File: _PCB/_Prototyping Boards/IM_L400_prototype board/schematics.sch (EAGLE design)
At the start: 10 parts

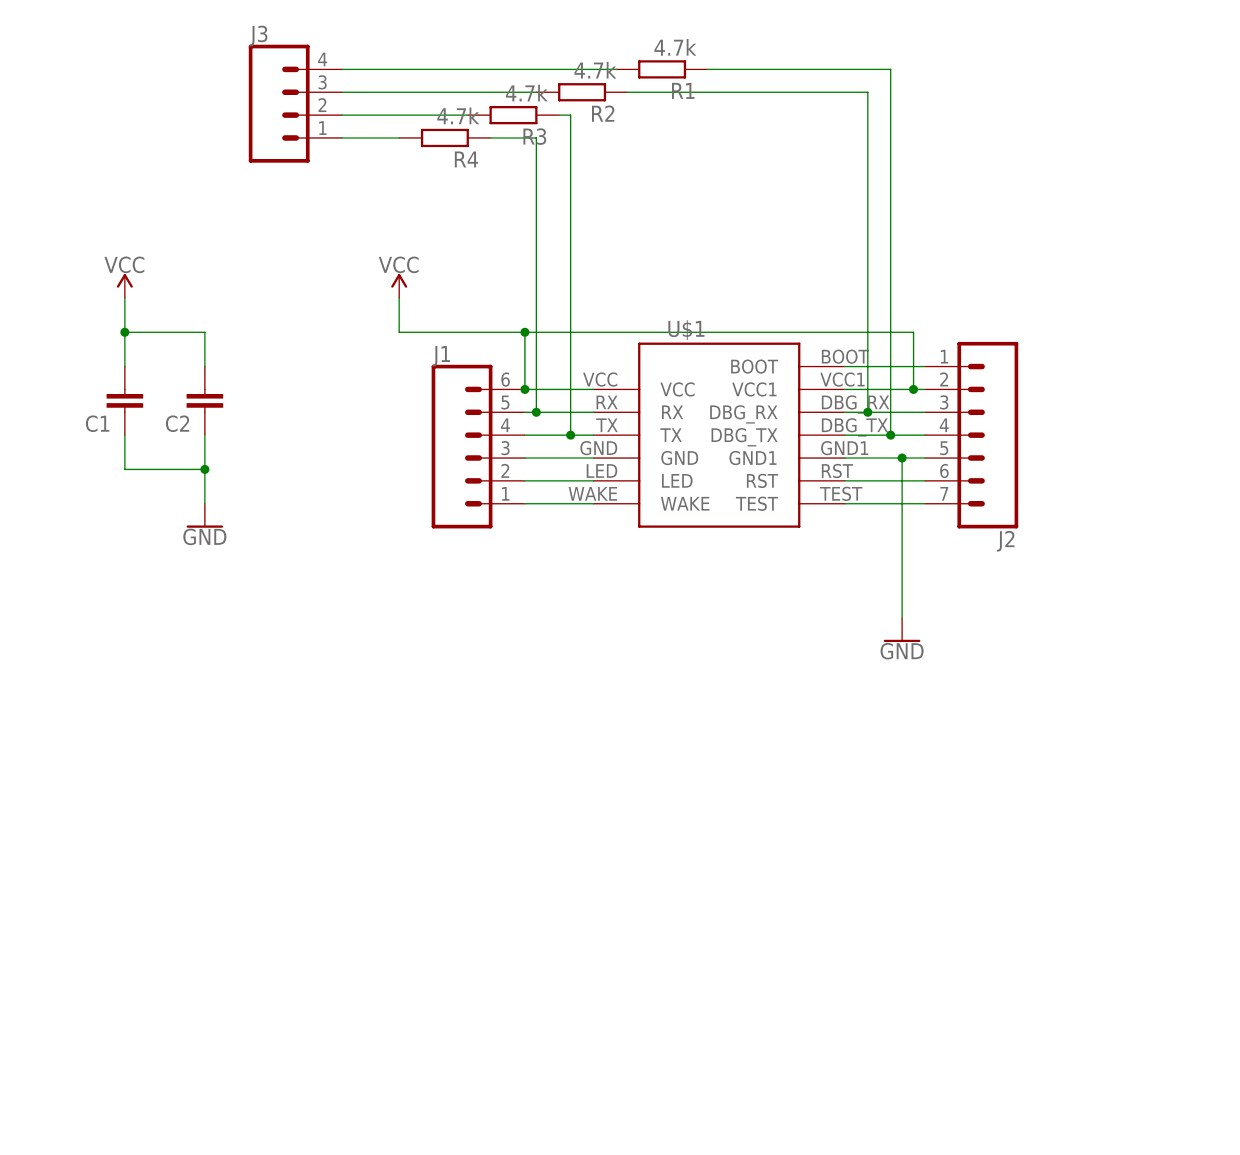
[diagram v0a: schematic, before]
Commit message: IM-L400 prototype board
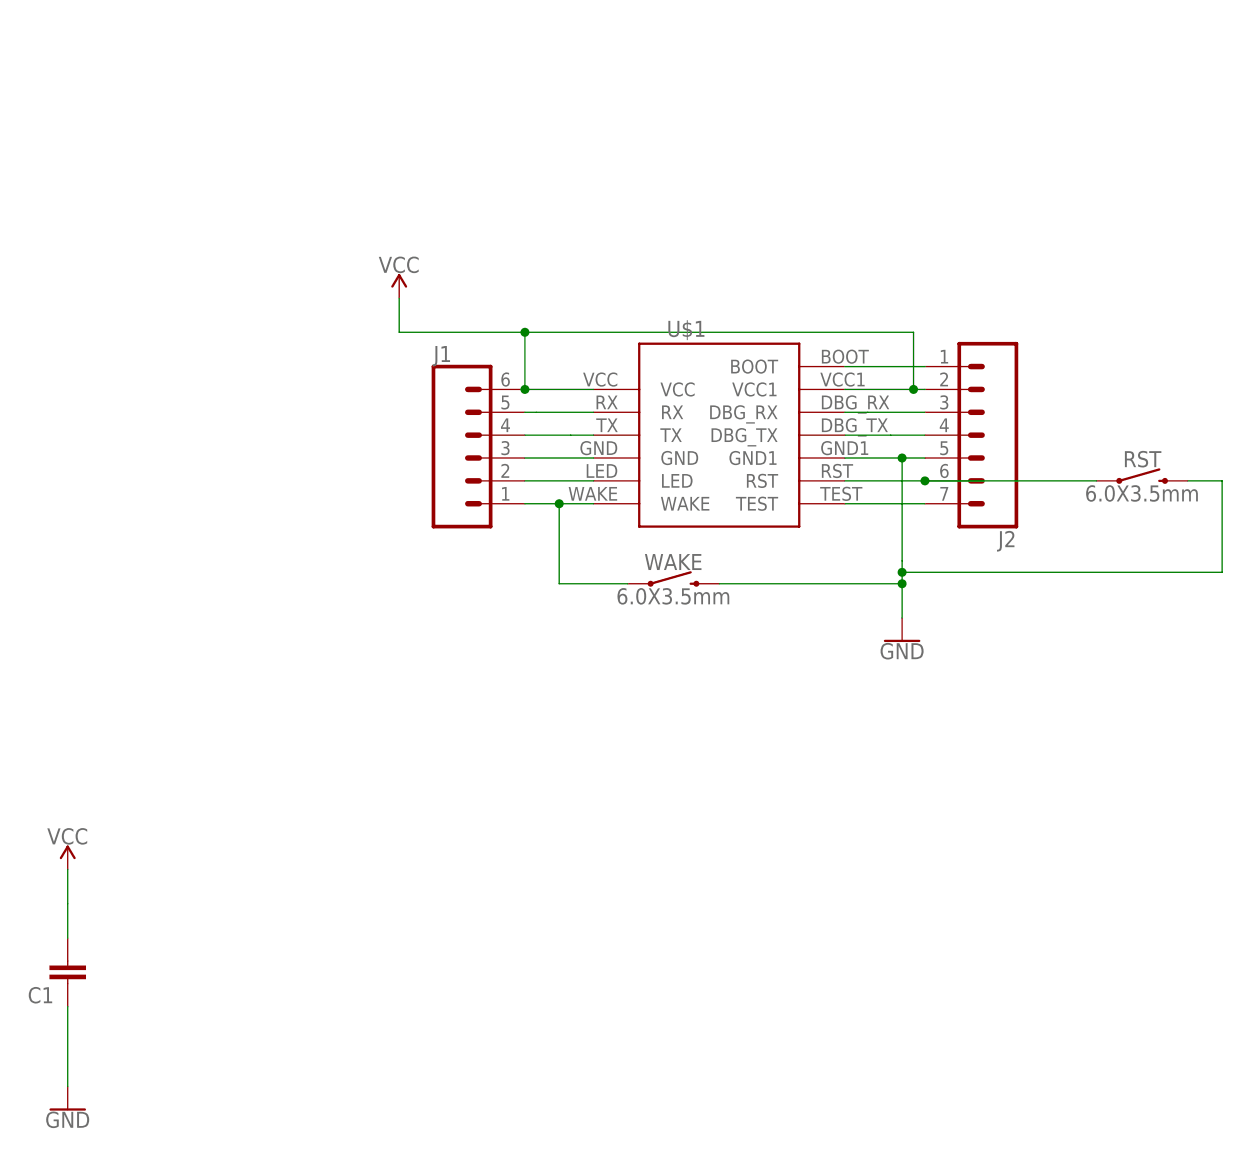
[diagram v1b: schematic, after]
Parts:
- removed C2: (no value), rcl:C-EUC0805
- removed J3: (no value), SparkFun-Connectors:CONN_04LOCK
- removed R1, R2, R3, R4: 4.7k, rcl:R-EU_R2012
- added RST, WAKE: 6.0X3.5mm, SparkFun-Switches:MOMENTARY-SWITCH-SPST-SMD-6.0X3.5MM
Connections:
- removed net N$14: J3.3, R2.2
- removed net N$15: J3.2, R3.2
- removed net N$16: J3.1, R4.2
- removed net N$4: J3.4, R1.2
- net GND: now also RST.2, WAKE.2; no longer C2.1
- net N$10: no longer R1.1
- net N$12: now also RST.1
- net N$2: no longer R4.1
- net N$3: no longer R3.1
- net N$6: now also WAKE.1
- net N$9: no longer R2.1
- net VCC: no longer C2.2
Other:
- moved on the sheet: C1
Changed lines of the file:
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@@
 <part name="J2" library="SparkFun-Connectors" library_urn="urn:adsk.eagle:library:513" deviceset="CONN_07" device="LOCK" package3d_urn="urn:adsk.eagle:package:38132/1"/>
 <part name="C1" library="rcl" library_urn="urn:adsk.eagle:library:334" deviceset="C-EU" device="C0805" package3d_urn="urn:adsk.eagle:package:23617/2"/>
-<part name="C2" library="rcl" library_urn="urn:adsk.eagle:library:334" deviceset="C-EU" device="C0805" package3d_urn="urn:adsk.eagle:package:23617/2"/>
-<part name="R1" library="rcl" library_urn="urn:adsk.eagle:library:334" deviceset="R-EU_" device="R2012" package3d_urn="urn:adsk.eagle:package:23543/2" value="4.7k"/>
-<part name="R2" library="rcl" library_urn="urn:adsk.eagle:library:334" deviceset="R-EU_" device="R2012" package3d_urn="urn:adsk.eagle:package:23543/2" value="4.7k"/>
-<part name="R3" library="rcl" library_urn="urn:adsk.eagle:library:334" deviceset="R-EU_" device="R2012" package3d_urn="urn:adsk.eagle:package:23543/2" value="4.7k"/>
-<part name="R4" library="rcl" library_urn="urn:adsk.eagle:library:334" deviceset="R-EU_" device="R2012" package3d_urn="urn:adsk.eagle:package:23543/2" value="4.7k"/>
-<part name="J3" library="SparkFun-Connectors" library_urn="urn:adsk.eagle:library:513" deviceset="CONN_04" device="LOCK" package3d_urn="urn:adsk.eagle:package:38089/1"/>
 <part name="GND1" library="SparkFun-PowerSymbols" library_urn="urn:adsk.eagle:library:530" deviceset="GND" device=""/>
 <part name="SUPPLY1" library="SparkFun-PowerSymbols" library_urn="urn:adsk.eagle:library:530" deviceset="VCC" device=""/>
 <part name="SUPPLY2" library="SparkFun-PowerSymbols" library_urn="urn:adsk.eagle:library:530" deviceset="VCC" device=""/>
 <part name="GND2" library="SparkFun-PowerSymbols" library_urn="urn:adsk.eagle:library:530" deviceset="GND" device=""/>
+<part name="WAKE" library="SparkFun-Switches" library_urn="urn:adsk.eagle:library:535" deviceset="MOMENTARY-SWITCH-SPST" device="-SMD-6.0X3.5MM" package3d_urn="urn:adsk.eagle:package:40165/1" value="6.0X3.5mm"/>
+<part name="RST" library="SparkFun-Switches" library_urn="urn:adsk.eagle:library:535" deviceset="MOMENTARY-SWITCH-SPST" device="-SMD-6.0X3.5MM" package3d_urn="urn:adsk.eagle:package:40165/1" value="6.0X3.5mm"/>
 </parts>
 <sheets>
@@
 <instance part="J1" gate="G$1" x="-2.54" y="12.7"/>
 <instance part="J2" gate="G$1" x="52.07" y="17.78" rot="R180"/>
-<instance part="C1" gate="G$1" x="-41.91" y="17.78" rot="R180"/>
-<instance part="C2" gate="G$1" x="-33.02" y="17.78" rot="R180"/>
-<instance part="R1" gate="G$1" x="17.78" y="55.88" rot="R180"/>
-<instance part="R2" gate="G$1" x="8.89" y="53.34" rot="R180"/>
-<instance part="R3" gate="G$1" x="1.27" y="50.8" rot="R180"/>
-<instance part="R4" gate="G$1" x="-6.35" y="48.26" rot="R180"/>
-<instance part="J3" gate="G$1" x="-22.86" y="50.8"/>
-<instance part="GND1" gate="1" x="-33.02" y="5.08"/>
-<instance part="SUPPLY1" gate="G$1" x="-41.91" y="30.48"/>
+<instance part="C1" gate="G$1" x="-48.26" y="-45.72" rot="R180"/>
+<instance part="GND1" gate="1" x="-48.26" y="-59.69"/>
+<instance part="SUPPLY1" gate="G$1" x="-48.26" y="-33.02"/>
 <instance part="SUPPLY2" gate="G$1" x="-11.43" y="30.48"/>
 <instance part="GND2" gate="1" x="44.45" y="-7.62"/>
+<instance part="WAKE" gate="G$1" x="19.05" y="-1.27"/>
+<instance part="RST" gate="G$1" x="71.12" y="10.16"/>
 </instances>
 <busses>
@@
 <pinref part="U$1" gate="G$1" pin="RX"/>
 <wire x1="2.54" y1="17.78" x2="3.81" y2="17.78" width="0.1524" layer="91"/>
-<pinref part="R4" gate="G$1" pin="1"/>
 <wire x1="3.81" y1="17.78" x2="10.16" y2="17.78" width="0.1524" layer="91"/>
-<wire x1="-1.27" y1="48.26" x2="3.81" y2="48.26" width="0.1524" layer="91"/>
-<wire x1="3.81" y1="48.26" x2="3.81" y2="17.78" width="0.1524" layer="91"/>
-<junction x="3.81" y="17.78"/>
 </segment>
 </net>
@@
 <pinref part="J1" gate="G$1" pin="4"/>
 <wire x1="10.16" y1="15.24" x2="7.62" y2="15.24" width="0.1524" layer="91"/>
-<pinref part="R3" gate="G$1" pin="1"/>
 <wire x1="7.62" y1="15.24" x2="2.54" y2="15.24" width="0.1524" layer="91"/>
-<wire x1="6.35" y1="50.8" x2="7.62" y2="50.8" width="0.1524" layer="91"/>
-<wire x1="7.62" y1="50.8" x2="7.62" y2="15.24" width="0.1524" layer="91"/>
-<junction x="7.62" y="15.24"/>
 </segment>
 </net>
@@
 </segment>
 <segment>
-<pinref part="C2" gate="G$1" pin="1"/>
-<pinref part="GND1" gate="1" pin="GND"/>
-<wire x1="-33.02" y1="15.24" x2="-33.02" y2="11.43" width="0.1524" layer="91"/>
-<pinref part="C1" gate="G$1" pin="1"/>
-<wire x1="-33.02" y1="11.43" x2="-33.02" y2="7.62" width="0.1524" layer="91"/>
-<wire x1="-41.91" y1="15.24" x2="-41.91" y2="11.43" width="0.1524" layer="91"/>
-<wire x1="-41.91" y1="11.43" x2="-33.02" y2="11.43" width="0.1524" layer="91"/>
-<junction x="-33.02" y="11.43"/>
-</segment>
-<segment>
 <pinref part="U$1" gate="G$1" pin="GND1"/>
 <pinref part="J2" gate="G$1" pin="5"/>
@@
 <pinref part="GND2" gate="1" pin="GND"/>
 <wire x1="44.45" y1="12.7" x2="46.99" y2="12.7" width="0.1524" layer="91"/>
-<wire x1="44.45" y1="12.7" x2="44.45" y2="-5.08" width="0.1524" layer="91"/>
+<wire x1="44.45" y1="12.7" x2="44.45" y2="1.27" width="0.1524" layer="91"/>
 <junction x="44.45" y="12.7"/>
+<wire x1="44.45" y1="1.27" x2="44.45" y2="0" width="0.1524" layer="91"/>
+<wire x1="44.45" y1="0" x2="44.45" y2="-1.27" width="0.1524" layer="91"/>
+<wire x1="44.45" y1="-1.27" x2="44.45" y2="-5.08" width="0.1524" layer="91"/>
+<pinref part="WAKE" gate="G$1" pin="2"/>
+<wire x1="24.13" y1="-1.27" x2="44.45" y2="-1.27" width="0.1524" layer="91"/>
+<junction x="44.45" y="-1.27"/>
+<pinref part="RST" gate="G$1" pin="2"/>
+<wire x1="76.2" y1="10.16" x2="80.01" y2="10.16" width="0.1524" layer="91"/>
+<wire x1="80.01" y1="10.16" x2="80.01" y2="0" width="0.1524" layer="91"/>
+<wire x1="80.01" y1="0" x2="44.45" y2="0" width="0.1524" layer="91"/>
+<junction x="44.45" y="0"/>
+</segment>
+<segment>
+<pinref part="C1" gate="G$1" pin="1"/>
+<pinref part="GND1" gate="1" pin="GND"/>
+<wire x1="-48.26" y1="-48.26" x2="-48.26" y2="-57.15" width="0.1524" layer="91"/>
 </segment>
 </net>
@@
 <pinref part="J1" gate="G$1" pin="1"/>
 <pinref part="U$1" gate="G$1" pin="WAKE"/>
-<wire x1="2.54" y1="7.62" x2="10.16" y2="7.62" width="0.1524" layer="91"/>
+<wire x1="2.54" y1="7.62" x2="6.35" y2="7.62" width="0.1524" layer="91"/>
+<pinref part="WAKE" gate="G$1" pin="1"/>
+<wire x1="6.35" y1="7.62" x2="10.16" y2="7.62" width="0.1524" layer="91"/>
+<wire x1="6.35" y1="7.62" x2="6.35" y2="-1.27" width="0.1524" layer="91"/>
+<wire x1="6.35" y1="-1.27" x2="13.97" y2="-1.27" width="0.1524" layer="91"/>
+<junction x="6.35" y="7.62"/>
 </segment>
 </net>
@@
 <pinref part="J2" gate="G$1" pin="3"/>
 <wire x1="38.1" y1="17.78" x2="40.64" y2="17.78" width="0.1524" layer="91"/>
-<pinref part="R2" gate="G$1" pin="1"/>
 <wire x1="40.64" y1="17.78" x2="46.99" y2="17.78" width="0.1524" layer="91"/>
-<wire x1="13.97" y1="53.34" x2="40.64" y2="53.34" width="0.1524" layer="91"/>
-<wire x1="40.64" y1="53.34" x2="40.64" y2="17.78" width="0.1524" layer="91"/>
-<junction x="40.64" y="17.78"/>
 </segment>
 </net>
@@
 <pinref part="U$1" gate="G$1" pin="DBG_TX"/>
 <wire x1="46.99" y1="15.24" x2="43.18" y2="15.24" width="0.1524" layer="91"/>
-<pinref part="R1" gate="G$1" pin="1"/>
 <wire x1="43.18" y1="15.24" x2="38.1" y2="15.24" width="0.1524" layer="91"/>
-<wire x1="22.86" y1="55.88" x2="43.18" y2="55.88" width="0.1524" layer="91"/>
-<wire x1="43.18" y1="55.88" x2="43.18" y2="15.24" width="0.1524" layer="91"/>
-<junction x="43.18" y="15.24"/>
 </segment>
 </net>
@@
 <pinref part="U$1" gate="G$1" pin="RST"/>
 <wire x1="46.99" y1="10.16" x2="38.1" y2="10.16" width="0.1524" layer="91"/>
+<pinref part="RST" gate="G$1" pin="1"/>
+<wire x1="66.04" y1="10.16" x2="46.99" y2="10.16" width="0.1524" layer="91"/>
+<junction x="46.99" y="10.16"/>
 </segment>
 </net>
@@
 <pinref part="C1" gate="G$1" pin="2"/>
 <pinref part="SUPPLY1" gate="G$1" pin="VCC"/>
-<wire x1="-41.91" y1="22.86" x2="-41.91" y2="26.67" width="0.1524" layer="91"/>
-<pinref part="C2" gate="G$1" pin="2"/>
-<wire x1="-41.91" y1="26.67" x2="-41.91" y2="30.48" width="0.1524" layer="91"/>
-<wire x1="-41.91" y1="26.67" x2="-33.02" y2="26.67" width="0.1524" layer="91"/>
-<wire x1="-33.02" y1="26.67" x2="-33.02" y2="22.86" width="0.1524" layer="91"/>
-<junction x="-41.91" y="26.67"/>
+<wire x1="-48.26" y1="-40.64" x2="-48.26" y2="-36.83" width="0.1524" layer="91"/>
+<wire x1="-48.26" y1="-36.83" x2="-48.26" y2="-33.02" width="0.1524" layer="91"/>
 </segment>
 <segment>
@@
 </segment>
 </net>
-<net name="N$4" class="0">
-<segment>
-<pinref part="R1" gate="G$1" pin="2"/>
-<pinref part="J3" gate="G$1" pin="4"/>
-<wire x1="12.7" y1="55.88" x2="-17.78" y2="55.88" width="0.1524" layer="91"/>
-</segment>
-</net>
-<net name="N$14" class="0">
-<segment>
-<pinref part="J3" gate="G$1" pin="3"/>
-<pinref part="R2" gate="G$1" pin="2"/>
-<wire x1="-17.78" y1="53.34" x2="3.81" y2="53.34" width="0.1524" layer="91"/>
-</segment>
-</net>
-<net name="N$15" class="0">
-<segment>
-<pinref part="R3" gate="G$1" pin="2"/>
-<pinref part="J3" gate="G$1" pin="2"/>
-<wire x1="-3.81" y1="50.8" x2="-17.78" y2="50.8" width="0.1524" layer="91"/>
-</segment>
-</net>
-<net name="N$16" class="0">
-<segment>
-<pinref part="J3" gate="G$1" pin="1"/>
-<pinref part="R4" gate="G$1" pin="2"/>
-<wire x1="-17.78" y1="48.26" x2="-11.43" y2="48.26" width="0.1524" layer="91"/>
-</segment>
-</net>
